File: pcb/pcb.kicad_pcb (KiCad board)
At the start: 2 copper layers, 129 x 93.3 mm, 53 parts, among them J1 MJ-4PP-9, SW1 SW_PUSH, SW10 SW_PUSH, SW11 SW_PUSH, SW12 SW_PUSH, SW13 SW_PUSH, SW14 SW_PUSH, SW15 SW_PUSH, SW16 SW_PUSH, SW17 SW_PUSH, SW18 SW_PUSH, SW2 SW_PUSH, SW3 SW_PUSH, SW4 SW_PUSH, SW5 SW_PUSH, SW6 SW_PUSH, SW7 SW_PUSH, SW8 SW_PUSH, SW9 SW_PUSH, U1 xiao-ble, U2 xiao-ble

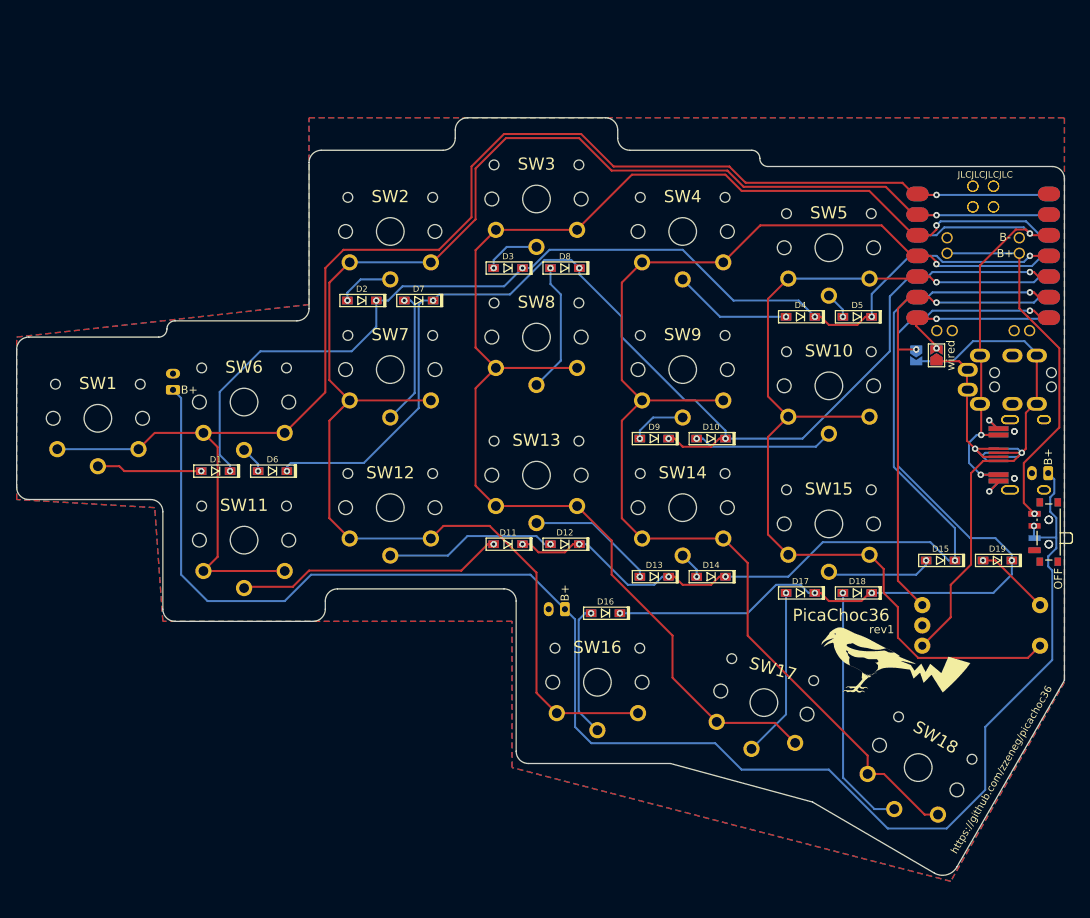
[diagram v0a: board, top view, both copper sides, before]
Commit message: small pcb
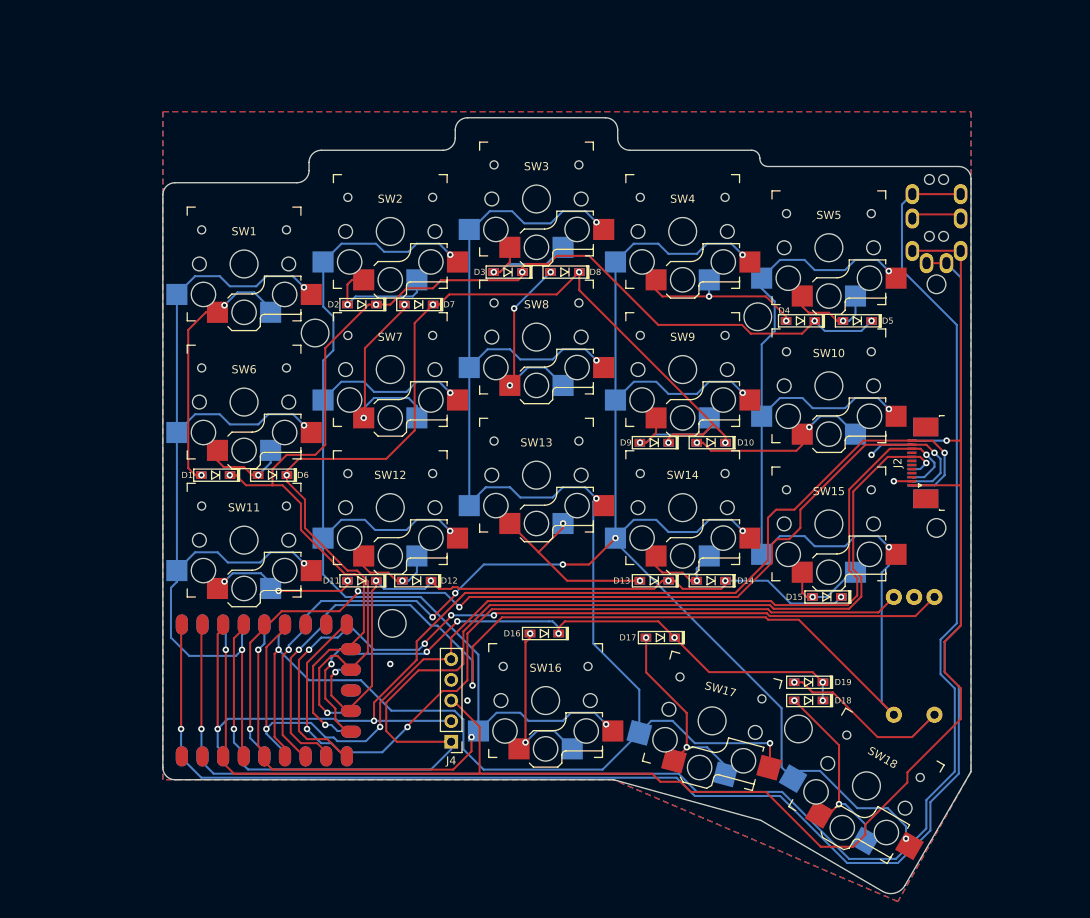
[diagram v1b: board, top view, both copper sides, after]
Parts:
- removed BATTCONN1, BATTCONN2, BATTCONN3: Conn_01x02_Female, picachoc:JST_PH_S2B-PH-K_1x02_P2.00mm
- removed BATTSW1, BATTSW2: SW_SPDT, Button_Switch_SMD:SW_SPDT_PCM12
- removed G***: LOGO, picachoc:logo
- removed G***: LOGO, picachoc:logo_mirror
- removed JP1, JP2, JP3: SolderJumper_2_Open, Jumper:SolderJumper-2_P1.3mm_Open_TrianglePad1.0x1.5mm
- removed USB1, USB2: HRO-TYPE-C-31-M-12, picachoc:HRO-TYPE-C-31-M-12-data
- added H1: MountingHole, picachoc:spacer_m2_3.4, F.Cu at (141.8, 67.5)
- added H2: MountingHole, picachoc:spacer_m2_3.4, F.Cu at (146.8, 118.2)
- added H3: MountingHole, picachoc:spacer_m2_3.4, F.Cu at (96.8, 105.2)
- added H4: MountingHole, picachoc:spacer_m2_3.4, F.Cu at (87.2, 69.5)
- added H5: MountingHole, kbd:thread_m2, F.Cu at (163.8, 93.5)
- added H6: MountingHole, kbd:thread_m2, F.Cu at (163.8, 63.5)
- added J2: Conn_01x12_Female, Connector_FFC-FPC:TE_1-1734839-2_1x12-1MP_P0.5mm_Horizontal, F.Cu at (162.1, 85.5)
- added J3: Conn_01x12_Female, Connector_FFC-FPC:TE_1-1734839-2_1x12-1MP_P0.5mm_Horizontal, B.Cu at (162.1, 85.5)
- added J4: Conn_01x05_Female, Connector_PinHeader_2.54mm:PinHeader_1x05_P2.54mm_Vertical, F.Cu at (104.0, 119.8)
- SW1, SW10, SW11, SW12, SW13, SW14, SW15, SW16, SW17, SW18, SW2, SW3, SW4, SW5, SW6, SW7, SW8, SW9: footprint picachoc:Kailh-PG1350-1u -> picachoc:Kailh_PG1350_hotswap
- U1, U2: value xiao-ble -> rp2040-zero; footprint picachoc:xiao-ble-smd -> picachoc:rp2040-zero-smd
- moved U1 103.4 mm to (81.0, 113.5), turned to -90 degrees
- moved U2 103.4 mm to (81.0, 113.5), turned to 90 degrees
- moved J1 30.5 mm to (163.8, 49.1), turned to 0 degrees
- moved D19 27.7 mm to (148.0, 112.5)
- moved SW1 26.2 mm to (78.5, 61.0)
- moved D12 18.8 mm to (99.8, 100.0)
- moved D11 18.6 mm to (93.0, 100.0)
- moved D17 18.1 mm to (129.8, 107.0)
- moved D15 14.7 mm to (150.2, 102.0)
- moved D18 14.5 mm to (148.0, 114.8)
- moved RE1 9.39 mm to (161.0, 109.5), turned to -90 degrees
- moved D16 7.93 mm to (115.5, 106.5)
- moved SW16 6.76 mm to (115.6, 114.8)
- moved SW17 6.76 mm to (136.1, 117.2)
- moved SW18 6.76 mm to (155.1, 125.2)
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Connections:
- J1 pad A: DATA -> TX
- J1 pad B: ENCB -> RX
- RE1 pad S1: SW_ENCB -> col4
- SW10 pad 2: SW_ENCB -> col4
- SW15 pad 2: SW_ENCB -> col4
- SW5 pad 2: SW_ENCB -> col4
- U1 pad 1: col0 -> TX
- U1 pad 10: row1 -> row0
- U1 pad 11: row0 -> row1
- U1 pad 12: VCC -> unconnected-(U1-Pad12)
- U1 pad 13: GND -> row2
- U1 pad 14: unconnected-(U1-Pad14) -> row3
- U1 pad 15: unconnected-(U1-Pad15) -> ENCA
- U1 pad 16: unconnected-(U1-Pad16) -> col4
- U1 pad 17: unconnected-(U1-Pad17) -> col3
- U1 pad 18: unconnected-(U1-Pad18) -> col2
- U1 pad 19: RAW -> col1
- U1 pad 2: col1 -> RX
- U1 pad 20: GND -> col0
- U1 pad 21: unconnected-(U1-Pad21) -> VCC
- U1 pad 22: unconnected-(U1-Pad22) -> GND
- U1 pad 3: col2 -> SCK
- U1 pad 4: col3 -> MOSI
- U1 pad 5: SW_ENCB -> MISO
- U1 pad 6: ENCA -> CS
- U1 pad 7: PIN7 -> unconnected-(U1-Pad7)
- U1 pad 8: row3 -> unconnected-(U1-Pad8)
- U1 pad 9: row2 -> ENCB
- U2 pad 1: col0 -> TX
- U2 pad 10: row1 -> row0
- U2 pad 11: row0 -> row1
- U2 pad 12: VCC -> unconnected-(U2-Pad12)
- U2 pad 13: GND -> row2
- U2 pad 14: unconnected-(U2-Pad14) -> row3
- U2 pad 15: unconnected-(U2-Pad15) -> ENCA
- U2 pad 16: unconnected-(U2-Pad16) -> col4
- U2 pad 17: unconnected-(U2-Pad17) -> col3
- U2 pad 18: unconnected-(U2-Pad18) -> col2
- U2 pad 19: RAW -> col1
- U2 pad 2: col1 -> RX
- U2 pad 20: GND -> col0
- U2 pad 21: unconnected-(U2-Pad21) -> VCC
- U2 pad 22: unconnected-(U2-Pad22) -> GND
- U2 pad 3: col2 -> SCK
- U2 pad 4: col3 -> MOSI
- U2 pad 5: SW_ENCB -> MISO
- U2 pad 6: ENCA -> CS
- U2 pad 7: PIN7 -> unconnected-(U2-Pad7)
- U2 pad 8: row3 -> unconnected-(U2-Pad8)
- U2 pad 9: row2 -> ENCB
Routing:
- net col4: track 0.00 -> 221.2 mm, vias 0 -> 5
- net RX: track 0.00 -> 202.6 mm, vias 0 -> 1
- net BATT: track 195.7 -> 0.00 mm, vias 1 -> 0
- net TX: track 0.00 -> 191.2 mm, vias 0 -> 1
- net MOSI: track 0.00 -> 150.7 mm, vias 0 -> 2
- net VCC: track 62.3 -> 209.8 mm, vias 3 -> 2
- net SCK: track 0.00 -> 143.4 mm, vias 0 -> 3
- net CS: track 0.00 -> 132.9 mm, vias 0 -> 3
- net SW_ENCB: track 122.2 -> 0.00 mm, vias 1 -> 0
- net MISO: track 0.00 -> 120.1 mm, vias 0 -> 4
- net col0: track 182.9 -> 122.5 mm, vias 1 -> 4
- net col3: track 160.4 -> 209.6 mm, vias 1 -> 9
- net RAW: track 45.4 -> 0.00 mm, vias 1 -> 0
- net ENCA: track 60.2 -> 99.8 mm, vias 2 -> 4
- net col2: track 178.8 -> 212.0 mm, vias 1 -> 5
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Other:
- board size 129 x 93.3 mm -> 99.5 x 95.5 mm
- board text removed: "JLCJLCJLCJLC"
- board text removed: "OFF"
- board text removed: "PicaChoc36"
- board text removed: "https://github.com/zzeneg/picachoc36"
- board text removed: "no enc"
- board text removed: "rev1"
- board text removed: "wired"
- board text removed: "wireless"

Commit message: new version
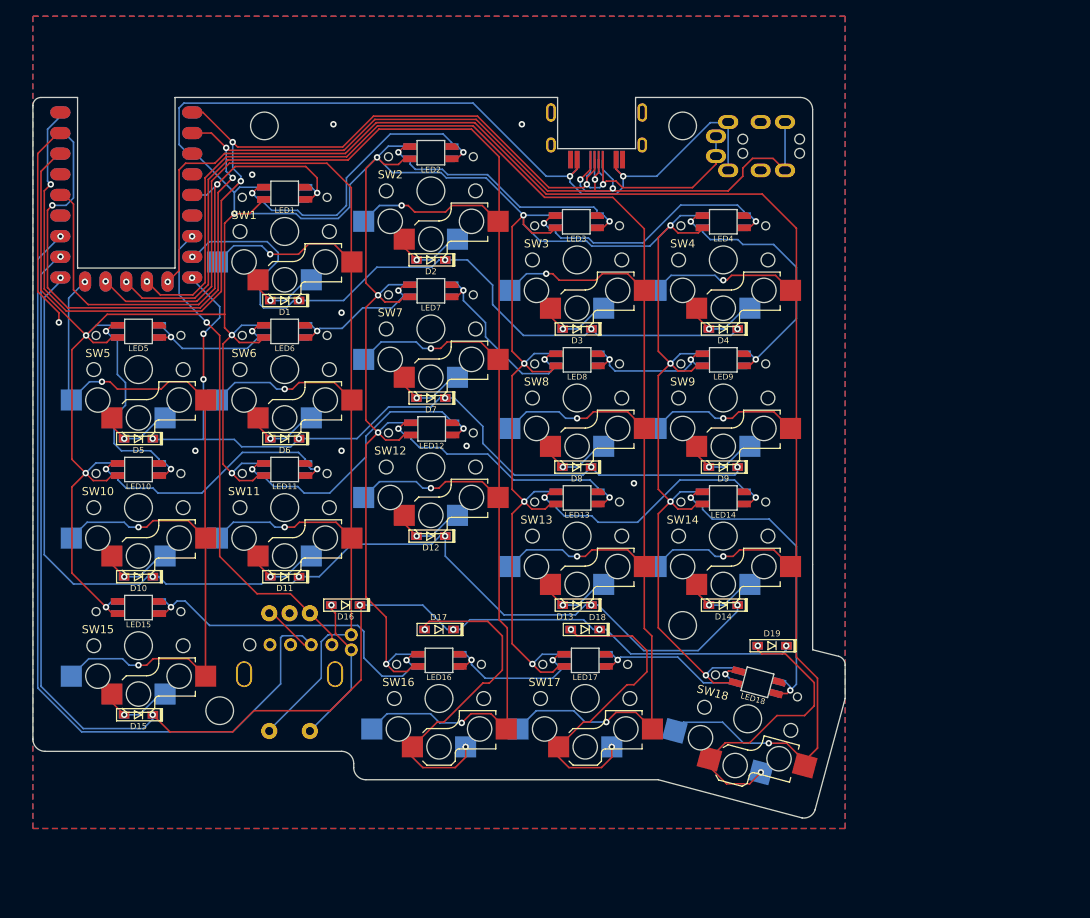
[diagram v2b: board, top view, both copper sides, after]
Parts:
- removed H5, H6: MountingHole, kbd:thread_m2
- removed J3: Conn_01x12_Female, Connector_FFC-FPC:TE_1-1734839-2_1x12-1MP_P0.5mm_Horizontal
- removed J4: Conn_01x05_Female, Connector_PinHeader_2.54mm:PinHeader_1x05_P2.54mm_Vertical
- added LED1: YS-SK6812MINI-E, zzkeeb:LED_SK6812-MINI-E-reversible, F.Cu at (83.5, 52.3)
- added LED10: YS-SK6812MINI-E, zzkeeb:LED_SK6812-MINI-E-reversible, F.Cu at (65.5, 86.3)
- added LED11: YS-SK6812MINI-E, zzkeeb:LED_SK6812-MINI-E-reversible, F.Cu at (83.5, 86.3)
- added LED12: YS-SK6812MINI-E, zzkeeb:LED_SK6812-MINI-E-reversible, F.Cu at (101.6, 81.3)
- added LED13: YS-SK6812MINI-E, zzkeeb:LED_SK6812-MINI-E-reversible, F.Cu at (119.5, 89.8)
- added LED14: YS-SK6812MINI-E, zzkeeb:LED_SK6812-MINI-E-reversible, F.Cu at (137.5, 89.8)
- added LED15: YS-SK6812MINI-E, zzkeeb:LED_SK6812-MINI-E-reversible, F.Cu at (65.5, 103.3)
- added LED16: YS-SK6812MINI-E, zzkeeb:LED_SK6812-MINI-E-reversible, F.Cu at (102.5, 109.8)
- added LED17: YS-SK6812MINI-E, zzkeeb:LED_SK6812-MINI-E-reversible, F.Cu at (120.5, 109.8)
- added LED18: YS-SK6812MINI-E, zzkeeb:LED_SK6812-MINI-E-reversible, F.Cu at (141.7, 112.5)
- added LED2: YS-SK6812MINI-E, zzkeeb:LED_SK6812-MINI-E-reversible, F.Cu at (101.5, 47.3)
- added LED3: YS-SK6812MINI-E, zzkeeb:LED_SK6812-MINI-E-reversible, F.Cu at (119.4, 55.8)
- added LED4: YS-SK6812MINI-E, zzkeeb:LED_SK6812-MINI-E-reversible, F.Cu at (137.5, 55.8)
- added LED5: YS-SK6812MINI-E, zzkeeb:LED_SK6812-MINI-E-reversible, F.Cu at (65.5, 69.3)
- added LED6: YS-SK6812MINI-E, zzkeeb:LED_SK6812-MINI-E-reversible, F.Cu at (83.5, 69.3)
- added LED7: YS-SK6812MINI-E, zzkeeb:LED_SK6812-MINI-E-reversible, F.Cu at (101.5, 64.3)
- added LED8: YS-SK6812MINI-E, zzkeeb:LED_SK6812-MINI-E-reversible, F.Cu at (119.5, 72.8)
- added LED9: YS-SK6812MINI-E, zzkeeb:LED_SK6812-MINI-E-reversible, F.Cu at (137.5, 72.8)
- added U3: roller, zzkeeb:RotaryEncoder_EVQWGD001, F.Cu at (85.5, 113.5)
- D1, D10, D11, D12, D13, D14, D15, D16, D17, D18, D19, D2, D3, D4, D5, D6, D7, D8, D9: footprint picachoc:D3_SMD -> zzkeeb:Diode_1N4148-SOD123-reversible; moved to B.Cu
- H1, H2, H3, H4: footprint picachoc:spacer_m2_3.4 -> zzkeeb:Hole_M2-spacer
- J1: footprint picachoc:MJ-4PP-9 -> zzkeeb:Connector_TRRS-reversible
- J2: value Conn_01x12_Female -> USB_C_Receptacle_USB2.0; footprint Connector_FFC-FPC:TE_1-1734839-2_1x12-1MP_P0.5mm_Horizontal -> zzkeeb:Connector_USB-C-mid-mount-ali-reversible-data
- RE1: footprint picachoc:RotaryEncoder_EC11 -> zzkeeb:RotaryEncoder_EC11
- SW1, SW10, SW11, SW12, SW13, SW14, SW15, SW16, SW17, SW18, SW2, SW3, SW4, SW5, SW6, SW7, SW8, SW9: footprint picachoc:Kailh_PG1350_hotswap -> zzkeeb:Switch_ChocV1-hotswap-reversible
- U1, U2: footprint picachoc:rp2040-zero-smd -> zzkeeb:MCU_rp2040-zero-smd
- moved D5 89.7 mm to (65.5, 82.5)
- moved SW10 86.3 mm to (65.5, 91.0)
- moved SW15 86.3 mm to (65.5, 108.0)
- moved SW5 86.3 mm to (65.5, 74.0)
- moved D15 86.0 mm to (65.5, 116.5)
- moved RE1 76.9 mm to (84.1, 111.5)
- moved D10 72.4 mm to (65.5, 99.5)
- moved U1 63.3 mm to (64.0, 52.5), turned to 180 degrees
- moved U2 63.3 mm to (64.0, 52.5), turned to 0 degrees
- moved J2 57.0 mm to (121.9, 45.0), turned to 180 degrees
- moved D18 28.9 mm to (120.5, 106.0)
- moved D17 27.3 mm to (102.5, 106.0)
- moved H4 26.3 mm to (81.0, 44.0)
- moved H1 25.3 mm to (132.5, 44.0)
- moved D16 24.7 mm to (91.0, 103.0)
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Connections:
- D10 pad 1: row1 -> row2
- D15 pad 1: row2 -> row3
- D16 pad 2: Net-(D16-Pad2) -> SW_ENCA
- D19 pad 2: SW_ENCA -> Net-(D19-Pad2)
- D5 pad 1: row0 -> row1
- RE1 pad S1: col4 -> col1
- SW1 pad 2: col0 -> col1
- SW10 pad 2: col4 -> col0
- SW11 pad 2: col0 -> col1
- SW12 pad 2: col1 -> col2
- SW13 pad 2: col2 -> col3
- SW14 pad 2: col3 -> col4
- SW15 pad 2: col4 -> col0
- SW16 pad 1: Net-(D16-Pad2) -> Net-(D17-Pad2)
- SW16 pad 2: col1 -> col2
- SW17 pad 1: Net-(D17-Pad2) -> Net-(D18-Pad2)
- SW17 pad 2: col2 -> col3
- SW18 pad 1: Net-(D18-Pad2) -> Net-(D19-Pad2)
- SW18 pad 2: col3 -> col4
- SW2 pad 2: col1 -> col2
- SW3 pad 2: col2 -> col3
- SW4 pad 2: col3 -> col4
- SW5 pad 2: col4 -> col0
- SW6 pad 2: col0 -> col1
- SW7 pad 2: col1 -> col2
- SW8 pad 2: col2 -> col3
- SW9 pad 2: col3 -> col4
- U1 pad 10: row0 -> col0
- U1 pad 11: row1 -> col1
- U1 pad 12: unconnected-(U1-Pad12) -> col2
- U1 pad 13: row2 -> col3
- U1 pad 14: row3 -> col4
- U1 pad 15: ENCA -> row1
- U1 pad 16: col4 -> row0
- U1 pad 17: col3 -> ENCA
- U1 pad 18: col2 -> unconnected-(U1-Pad18)
- U1 pad 19: col1 -> LED
- U1 pad 20: col0 -> unconnected-(U1-Pad20)
- U1 pad 3: SCK -> unconnected-(U1-Pad3)
- U1 pad 4: MOSI -> unconnected-(U1-Pad4)
- U1 pad 5: MISO -> unconnected-(U1-Pad5)
- U1 pad 6: CS -> unconnected-(U1-Pad6)
- U1 pad 7: unconnected-(U1-Pad7) -> ENCB
- U1 pad 8: unconnected-(U1-Pad8) -> row3
- U1 pad 9: ENCB -> row2
- U2 pad 10: row0 -> col4
- U2 pad 11: row1 -> col3
- U2 pad 12: unconnected-(U2-Pad12) -> col2
- U2 pad 13: row2 -> col1
- U2 pad 14: row3 -> col0
- U2 pad 15: ENCA -> row2
- U2 pad 16: col4 -> row3
- U2 pad 17: col3 -> ENCB
- U2 pad 18: col2 -> unconnected-(U2-Pad18)
- U2 pad 19: col1 -> LED
- U2 pad 20: col0 -> unconnected-(U2-Pad20)
- U2 pad 3: SCK -> unconnected-(U2-Pad3)
- U2 pad 4: MOSI -> unconnected-(U2-Pad4)
- U2 pad 5: MISO -> unconnected-(U2-Pad5)
- U2 pad 6: CS -> unconnected-(U2-Pad6)
- U2 pad 7: unconnected-(U2-Pad7) -> ENCA
- U2 pad 8: unconnected-(U2-Pad8) -> row0
- U2 pad 9: ENCB -> row1
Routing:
- net VCC: track 209.8 -> 634.0 mm, vias 2 -> 20
- net MOSI: track 150.7 -> 0.00 mm, vias 2 -> 0
- net SCK: track 143.4 -> 0.00 mm, vias 3 -> 0
- net CS: track 132.9 -> 0.00 mm, vias 3 -> 0
- net MISO: track 120.1 -> 0.00 mm, vias 4 -> 0
- net row3: track 80.9 -> 166.0 mm, vias 7 -> 6
- net LED: track 0.00 -> 67.4 mm, vias 0 -> 2
- net row0: track 148.7 -> 87.3 mm, vias 6 -> 5
- net row2: track 86.7 -> 136.0 mm
- net Net-(LED15-Pad4): track 0.00 -> 44.0 mm, vias 0 -> 2
- net Net-(LED14-Pad2): track 0.00 -> 39.7 mm, vias 0 -> 2
- net ENCA: track 99.8 -> 61.1 mm, vias 4 -> 2
- net Net-(LED1-Pad2): track 0.00 -> 38.3 mm, vias 0 -> 2
- net Net-(LED11-Pad2): track 0.00 -> 37.3 mm, vias 0 -> 2
- net Net-(D19-Pad2): track 0.00 -> 36.4 mm, vias 0 -> 2
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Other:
- board size 99.5 x 95.5 mm -> 100 x 88.7 mm
